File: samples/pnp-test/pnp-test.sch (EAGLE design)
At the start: 38 parts

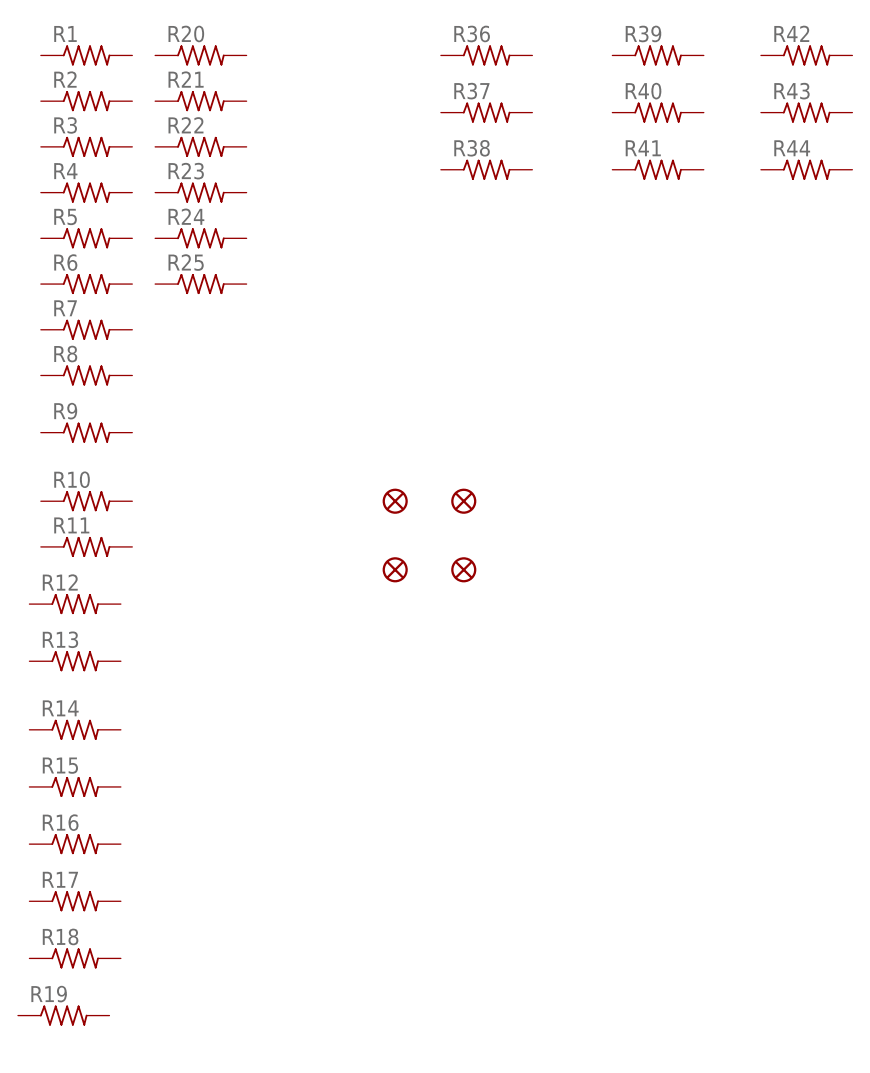
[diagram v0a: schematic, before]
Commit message: Put together a full demo suite. Fresh install now boots clean and can immediately run the pnp-test job.
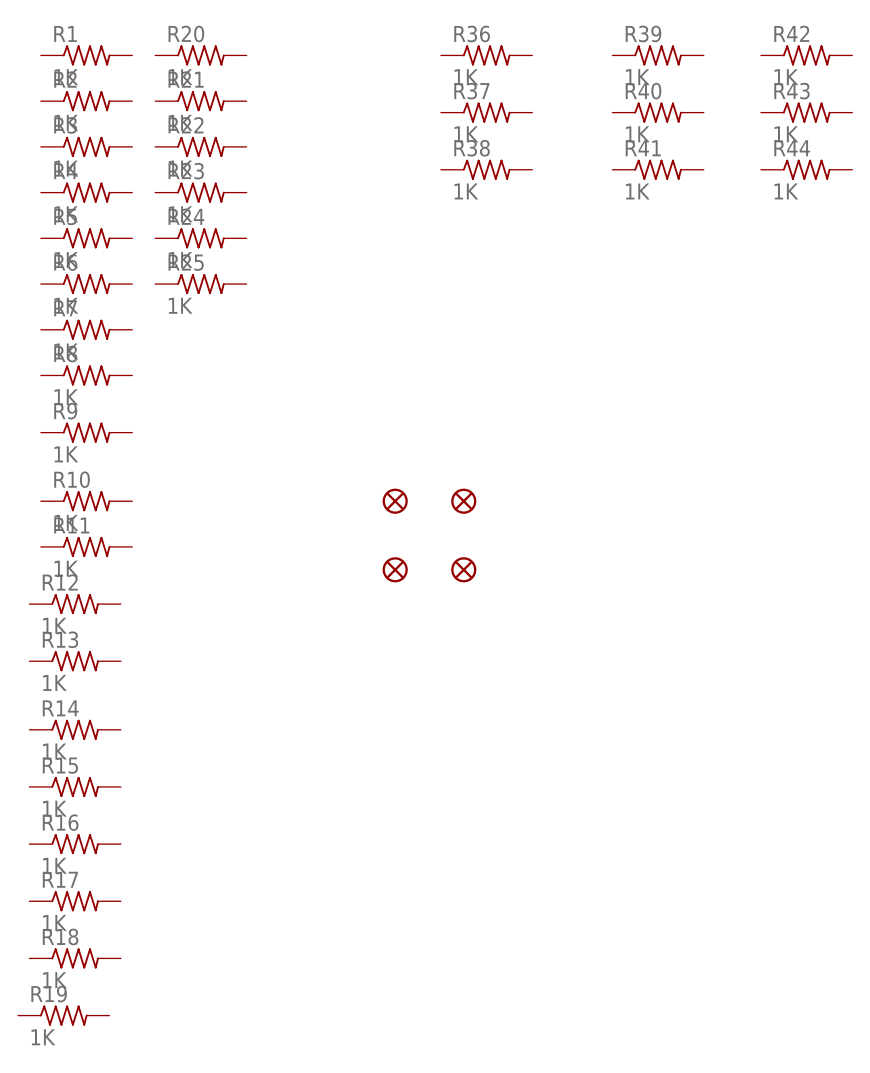
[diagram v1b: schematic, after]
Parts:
- R1, R10, R11, R12, R13, R14, R15, R16, R17, R18, R19, R2, R20, R21, R22, R23, R24, R25, R3, R36, R37, R38, R39, R4, R40, R41, R42, R43, R44, R5, R6, R7, R8, R9: value (none) -> 1K
- renumbered U$1 to FID1, U$2 to FID2, U$3 to FID3, U$4 to FID4
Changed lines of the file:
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@@
 </classes>
 <parts>
-<part name="R1" library="rcl" deviceset="R-US_" device="R0805"/>
-<part name="R2" library="rcl" deviceset="R-US_" device="R0805"/>
-<part name="R3" library="rcl" deviceset="R-US_" device="R0805"/>
-<part name="R4" library="rcl" deviceset="R-US_" device="R0805"/>
-<part name="R5" library="rcl" deviceset="R-US_" device="R0805"/>
-<part name="R6" library="rcl" deviceset="R-US_" device="R0805"/>
-<part name="R7" library="rcl" deviceset="R-US_" device="R0805"/>
-<part name="R8" library="rcl" deviceset="R-US_" device="R0805"/>
-<part name="R9" library="rcl" deviceset="R-US_" device="R0805"/>
-<part name="R10" library="rcl" deviceset="R-US_" device="R0805"/>
-<part name="R11" library="rcl" deviceset="R-US_" device="R0805"/>
-<part name="R12" library="rcl" deviceset="R-US_" device="R0805"/>
-<part name="R13" library="rcl" deviceset="R-US_" device="R0805"/>
-<part name="R14" library="rcl" deviceset="R-US_" device="R0805"/>
-<part name="R15" library="rcl" deviceset="R-US_" device="R0805"/>
-<part name="R16" library="rcl" deviceset="R-US_" device="R0805"/>
-<part name="R17" library="rcl" deviceset="R-US_" device="R0805"/>
-<part name="R18" library="rcl" deviceset="R-US_" device="R0805"/>
-<part name="R19" library="rcl" deviceset="R-US_" device="R0805"/>
-<part name="R20" library="rcl" deviceset="R-US_" device="R0805"/>
-<part name="R21" library="rcl" deviceset="R-US_" device="R0805"/>
-<part name="R22" library="rcl" deviceset="R-US_" device="R0805"/>
-<part name="R23" library="rcl" deviceset="R-US_" device="R0805"/>
-<part name="R24" library="rcl" deviceset="R-US_" device="R0805"/>
-<part name="R25" library="rcl" deviceset="R-US_" device="R0805"/>
-<part name="R36" library="rcl" deviceset="R-US_" device="R0201"/>
-<part name="R37" library="rcl" deviceset="R-US_" device="R0201"/>
-<part name="R38" library="rcl" deviceset="R-US_" device="R0201"/>
-<part name="R39" library="rcl" deviceset="R-US_" device="R0402"/>
-<part name="R40" library="rcl" deviceset="R-US_" device="R0402"/>
-<part name="R41" library="rcl" deviceset="R-US_" device="R0402"/>
-<part name="R42" library="rcl" deviceset="R-US_" device="R0603"/>
-<part name="R43" library="rcl" deviceset="R-US_" device="R0603"/>
-<part name="R44" library="rcl" deviceset="R-US_" device="R0603"/>
-<part name="U$1" library="SparkFun" deviceset="FIDUCIAL" device="1X2"/>
-<part name="U$2" library="SparkFun" deviceset="FIDUCIAL" device="1X2"/>
-<part name="U$3" library="SparkFun" deviceset="FIDUCIAL" device="1X2"/>
-<part name="U$4" library="SparkFun" deviceset="FIDUCIAL" device="1X2"/>
+<part name="R1" library="rcl" deviceset="R-US_" device="R0805" value="1K"/>
+<part name="R2" library="rcl" deviceset="R-US_" device="R0805" value="1K"/>
+<part name="R3" library="rcl" deviceset="R-US_" device="R0805" value="1K"/>
+<part name="R4" library="rcl" deviceset="R-US_" device="R0805" value="1K"/>
+<part name="R5" library="rcl" deviceset="R-US_" device="R0805" value="1K"/>
+<part name="R6" library="rcl" deviceset="R-US_" device="R0805" value="1K"/>
+<part name="R7" library="rcl" deviceset="R-US_" device="R0805" value="1K"/>
+<part name="R8" library="rcl" deviceset="R-US_" device="R0805" value="1K"/>
+<part name="R9" library="rcl" deviceset="R-US_" device="R0805" value="1K"/>
+<part name="R10" library="rcl" deviceset="R-US_" device="R0805" value="1K"/>
+<part name="R11" library="rcl" deviceset="R-US_" device="R0805" value="1K"/>
+<part name="R12" library="rcl" deviceset="R-US_" device="R0805" value="1K"/>
+<part name="R13" library="rcl" deviceset="R-US_" device="R0805" value="1K"/>
+<part name="R14" library="rcl" deviceset="R-US_" device="R0805" value="1K"/>
+<part name="R15" library="rcl" deviceset="R-US_" device="R0805" value="1K"/>
+<part name="R16" library="rcl" deviceset="R-US_" device="R0805" value="1K"/>
+<part name="R17" library="rcl" deviceset="R-US_" device="R0805" value="1K"/>
+<part name="R18" library="rcl" deviceset="R-US_" device="R0805" value="1K"/>
+<part name="R19" library="rcl" deviceset="R-US_" device="R0805" value="1K"/>
+<part name="R20" library="rcl" deviceset="R-US_" device="R0805" value="1K"/>
+<part name="R21" library="rcl" deviceset="R-US_" device="R0805" value="1K"/>
+<part name="R22" library="rcl" deviceset="R-US_" device="R0805" value="1K"/>
+<part name="R23" library="rcl" deviceset="R-US_" device="R0805" value="1K"/>
+<part name="R24" library="rcl" deviceset="R-US_" device="R0805" value="1K"/>
+<part name="R25" library="rcl" deviceset="R-US_" device="R0805" value="1K"/>
+<part name="R36" library="rcl" deviceset="R-US_" device="R0201" value="1K"/>
+<part name="R37" library="rcl" deviceset="R-US_" device="R0201" value="1K"/>
+<part name="R38" library="rcl" deviceset="R-US_" device="R0201" value="1K"/>
+<part name="R39" library="rcl" deviceset="R-US_" device="R0402" value="1K"/>
+<part name="R40" library="rcl" deviceset="R-US_" device="R0402" value="1K"/>
+<part name="R41" library="rcl" deviceset="R-US_" device="R0402" value="1K"/>
+<part name="R42" library="rcl" deviceset="R-US_" device="R0603" value="1K"/>
+<part name="R43" library="rcl" deviceset="R-US_" device="R0603" value="1K"/>
+<part name="R44" library="rcl" deviceset="R-US_" device="R0603" value="1K"/>
+<part name="FID1" library="SparkFun" deviceset="FIDUCIAL" device="1X2"/>
+<part name="FID2" library="SparkFun" deviceset="FIDUCIAL" device="1X2"/>
+<part name="FID3" library="SparkFun" deviceset="FIDUCIAL" device="1X2"/>
+<part name="FID4" library="SparkFun" deviceset="FIDUCIAL" device="1X2"/>
 </parts>
 <sheets>
@@
 <instance part="R43" gate="G$1" x="43.18" y="137.16"/>
 <instance part="R44" gate="G$1" x="43.18" y="130.81"/>
-<instance part="U$1" gate="G$1" x="-2.54" y="86.36"/>
-<instance part="U$2" gate="G$1" x="5.08" y="86.36"/>
-<instance part="U$3" gate="G$1" x="5.08" y="93.98"/>
-<instance part="U$4" gate="G$1" x="-2.54" y="93.98"/>
+<instance part="FID1" gate="G$1" x="-2.54" y="86.36"/>
+<instance part="FID2" gate="G$1" x="5.08" y="86.36"/>
+<instance part="FID3" gate="G$1" x="5.08" y="93.98"/>
+<instance part="FID4" gate="G$1" x="-2.54" y="93.98"/>
 </instances>
 <busses>
